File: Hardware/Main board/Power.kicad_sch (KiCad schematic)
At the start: 14 parts, among them U5 AP7361C-33E, U6 AP7361C-33E, U7 AP7361C-33E, U8 AP7361C-33E, U9 TPM8837C

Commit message: Part selection
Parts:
- U5, U6, U7, U8: JLCPCB Part # (none) -> C500795; LCSC Part # (none) -> C500795
- U9: JLCPCB Part # (none) -> C7436831; LCSC Part # (none) -> C7436831
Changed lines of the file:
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@@
+			)
+		)
+		(property "JLCPCB Part #" "C500795"
+			(at 222.25 54.61 0)
+			(effects
+				(font
+					(size 1.27 1.27)
+				)
+				(hide yes)
+			)
+		)
+		(property "LCSC Part #" "C500795"
+			(at 222.25 54.61 0)
+			(effects
+				(font
+					(size 1.27 1.27)
+				)
+				(hide yes)
 			)
 		)
@@
 			)
 		)
+		(property "JLCPCB Part #" "C500795"
+			(at 168.91 64.77 0)
+			(effects
+				(font
+					(size 1.27 1.27)
+				)
+				(hide yes)
+			)
+		)
+		(property "LCSC Part #" "C500795"
+			(at 168.91 64.77 0)
+			(effects
+				(font
+					(size 1.27 1.27)
+				)
+				(hide yes)
+			)
+		)
 		(pin "3"
 		)
@@
 			)
 		)
+		(property "JLCPCB Part #" "C500795"
+			(at 62.23 64.77 0)
+			(effects
+				(font
+					(size 1.27 1.27)
+				)
+				(hide yes)
+			)
+		)
+		(property "LCSC Part #" "C500795"
+			(at 62.23 64.77 0)
+			(effects
+				(font
+					(size 1.27 1.27)
+				)
+				(hide yes)
+			)
+		)
 		(pin "3"
 		)
@@
 			)
 		)
+		(property "JLCPCB Part #" "C7436831"
+			(at 59.69 115.57 0)
+			(effects
+				(font
+					(size 1.27 1.27)
+				)
+				(hide yes)
+			)
+		)
+		(property "LCSC Part #" "C7436831"
+			(at 59.69 115.57 0)
+			(effects
+				(font
+					(size 1.27 1.27)
+				)
+				(hide yes)
+			)
+		)
 		(pin "8"
 		)
@@
 			(at 115.57 64.77 0)
 			(effects
+				(font
+					(size 1.27 1.27)
+				)
+				(hide yes)
+			)
+		)
+		(property "JLCPCB Part #" "C500795"
+			(at 115.57 64.77 0)
+			(effects
+				(font
+					(size 1.27 1.27)
+				)
+				(hide yes)
+			)
+		)
+		(property "LCSC Part #" "C500795"
+			(at 115.57 64.77 0)
+			(effects

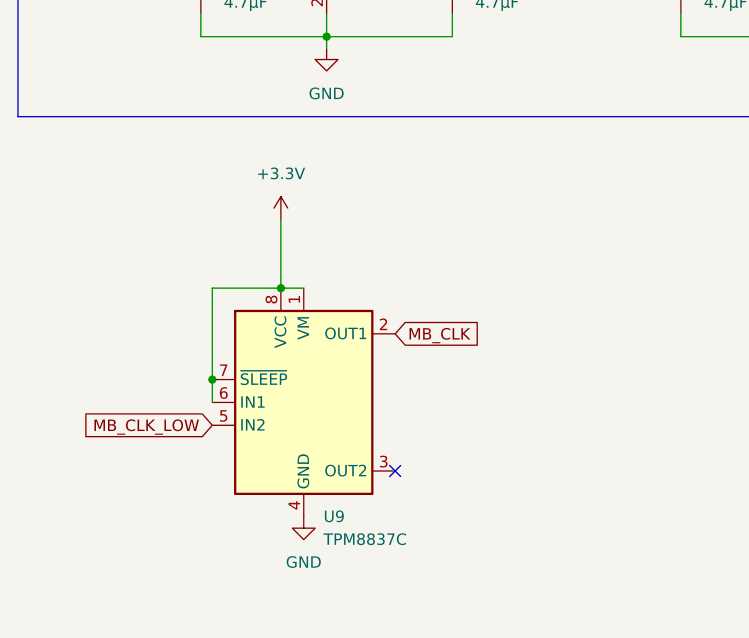
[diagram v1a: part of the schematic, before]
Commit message: Reworking BMS
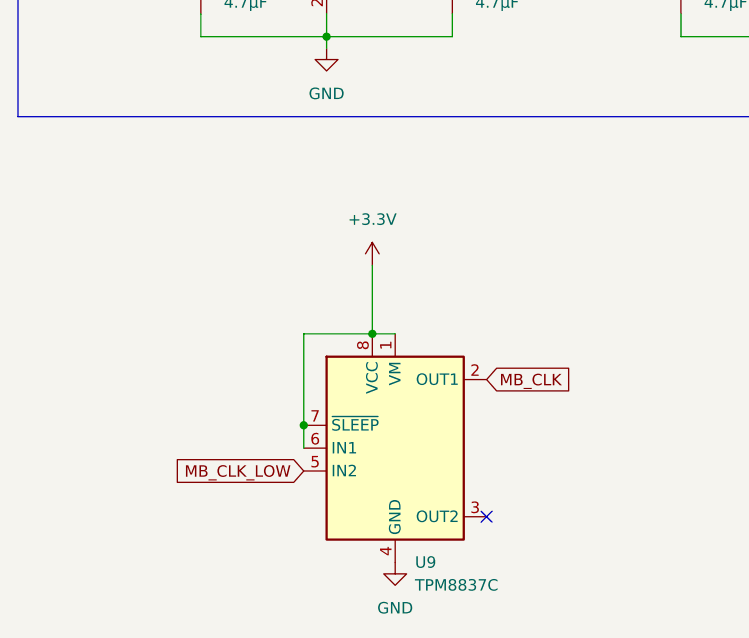
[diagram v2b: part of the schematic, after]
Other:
- moved on the sheet: U9
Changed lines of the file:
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@@
 	(paper "A4")
 	(junction
-		(at 49.53 113.03)
+		(at 59.69 118.11)
 		(diameter 0)
 		(color 0 0 0 0)
@@
 	)
 	(junction
-		(at 57.15 102.87)
+		(at 67.31 107.95)
 		(diameter 0)
 		(color 0 0 0 0)
@@
 	)
 	(no_connect
-		(at 69.85 123.19)
+		(at 80.01 128.27)
 	)
 	(wire
@@
 	(wire
 		(pts
-			(xy 49.53 113.03) (xy 49.53 115.57)
+			(xy 59.69 118.11) (xy 59.69 120.65)
 		)
 		(stroke
@@
 	(wire
 		(pts
-			(xy 57.15 95.25) (xy 57.15 102.87)
+			(xy 67.31 100.33) (xy 67.31 107.95)
 		)
 		(stroke
@@
 	(wire
 		(pts
-			(xy 57.15 102.87) (xy 59.69 102.87)
+			(xy 67.31 107.95) (xy 69.85 107.95)
 		)
 		(stroke
@@
 	(wire
 		(pts
-			(xy 49.53 102.87) (xy 49.53 113.03)
+			(xy 59.69 107.95) (xy 59.69 118.11)
 		)
 		(stroke
@@
 	(wire
 		(pts
-			(xy 57.15 102.87) (xy 49.53 102.87)
+			(xy 67.31 107.95) (xy 59.69 107.95)
 		)
 		(stroke
@@
 	(global_label "MB_CLK_LOW"
 		(shape input)
-		(at 49.53 118.11 180)
+		(at 59.69 123.19 180)
 		(fields_autoplaced yes)
 		(effects
@@
 		)
 		(property "Intersheetrefs" "${INTERSHEET_REFS}"
-			(at 34.5101 118.11 0)
+			(at 44.6701 123.19 0)
 			(effects
 				(font
@@
 	(global_label "MB_CLK"
 		(shape input)
-		(at 69.85 107.95 0)
+		(at 80.01 113.03 0)
 		(fields_autoplaced yes)
 		(effects
@@
 		)
 		(property "Intersheetrefs" "${INTERSHEET_REFS}"
-			(at 80.0923 107.95 0)
+			(at 90.2523 113.03 0)
 			(effects
 				(font
@@
 			)
 		)
+		(property "Design guide" ""
+			(at 101.6 69.85 0)
+			(effects
+				(font
+					(size 1.27 1.27)
+				)
+				(hide yes)
+			)
+		)
 		(pin "1"
 		)
@@
 			)
 		)
+		(property "Design guide" ""
+			(at 236.22 59.69 0)
+			(effects
+				(font
+					(size 1.27 1.27)
+				)
+				(hide yes)
+			)
+		)
 		(pin "1"
 		)
@@
 		)
 		(property "LCSC Part #" "C500795"
+			(at 222.25 54.61 0)
+			(effects
+				(font
+					(size 1.27 1.27)
+				)
+				(hide yes)
+			)
+		)
+		(property "Design guide" ""
 			(at 222.25 54.61 0)
 			(effects
@@
 			)
 		)
+		(property "Design guide" ""
+			(at 76.2 69.85 0)
+			(effects
+				(font
+					(size 1.27 1.27)
+				)
+				(hide yes)
+			)
+		)
 		(pin "1"
 		)
@@
 			)
 		)
+		(property "Design guide" ""
+			(at 48.26 69.85 0)
+			(effects
+				(font
+					(size 1.27 1.27)
+				)
+				(hide yes)
+			)
+		)
 		(pin "1"
 		)
@@
 	(symbol
 		(lib_id "power:+3.3V")
-		(at 57.15 95.25 0)
+		(at 67.31 100.33 0)
 		(unit 1)
 		(exclude_from_sim no)
@@
 		(fields_autoplaced yes)
 		(property "Reference" "#PWR044"
-			(at 57.15 99.06 0)
+			(at 67.31 104.14 0)
 			(effects
 				(font
@@
 		)
 		(property "Value" "+3.3V"
-			(at 57.15 90.17 0)
+			(at 67.31 95.25 0)
 			(effects
 				(font
@@
 		)
 		(property "Footprint" ""
-			(at 57.15 95.25 0)
+			(at 67.31 100.33 0)
 			(effects
 				(font
@@
 		)
 		(property "Datasheet" ""
-			(at 57.15 95.25 0)
+			(at 67.31 100.33 0)
 			(effects
 				(font
@@
 		)
 		(property "Description" "Power symbol creates a global label with name \"+3.3V\""
-			(at 57.15 95.25 0)
+			(at 67.31 100.33 0)
 			(effects
 				(font
@@
 			)
 		)
+		(property "Design guide" ""
+			(at 48.26 49.53 0)
+			(effects
+				(font
+					(size 1.27 1.27)
+				)
+				(hide yes)
+			)
+		)
 		(pin "1"
 		)
@@
 			)
 		)
+		(property "Design guide" ""
+			(at 208.28 59.69 0)
+			(effects
+				(font
+					(size 1.27 1.27)
+				)
+				(hide yes)
+			)
+		)
 		(pin "1"
 		)
@@
 			)
 		)
+		(property "Design guide" ""
+			(at 168.91 64.77 0)
+			(effects
+				(font
+					(size 1.27 1.27)
+				)
+				(hide yes)
+			)
+		)
 		(pin "3"
 		)
@@
 			)
 		)
+		(property "Design guide" ""
+			(at 182.88 69.85 0)
+			(effects
+				(font
+					(size 1.27 1.27)
+				)
+				(hide yes)
+			)
+		)
 		(pin "1"
 		)
@@
 			)
 		)
+		(property "Design guide" ""
+			(at 62.23 64.77 0)
+			(effects
+				(font
+					(size 1.27 1.27)
+				)
+				(hide yes)
+			)
+		)
 		(pin "3"
 		)
@@
 	(symbol
 		(lib_id "power:GND")
-		(at 59.69 128.27 0)
+		(at 69.85 133.35 0)
 		(unit 1)
 		(exclude_from_sim no)
@@
 		(fields_autoplaced yes)
 		(property "Reference" "#PWR045"
-			(at 59.69 134.62 0)
+			(at 69.85 139.7 0)
 			(effects
 				(font
@@
 		)
 		(property "Value" "GND"
-			(at 59.69 133.35 0)
+			(at 69.85 138.43 0)
 			(effects
 				(font
@@
 		)
 		(property "Footprint" ""
-			(at 59.69 128.27 0)
+			(at 69.85 133.35 0)
 			(effects
 				(font
@@
 		)
 		(property "Datasheet" ""
-			(at 59.69 128.27 0)
+			(at 69.85 133.35 0)
 			(effects
 				(font
@@
 		)
 		(property "Description" "Power symbol creates a global label with name \"GND\" , ground"
-			(at 59.69 128.27 0)
+			(at 69.85 133.35 0)
 			(effects
 				(font
@@
 			)
 		)
+		(property "Design guide" ""
+			(at 129.54 69.85 0)
+			(effects
+				(font
+					(size 1.27 1.27)
+				)
+				(hide yes)
+			)
+		)
 		(pin "1"
 		)
@@
 	(symbol
 		(lib_id "Driver_Motor:DRV8837C")
-		(at 59.69 115.57 0)
+		(at 69.85 120.65 0)
 		(unit 1)
 		(exclude_from_sim no)
@@
 		(dnp no)
 		(property "Reference" "U9"
-			(at 61.8841 128.27 0)
+			(at 72.0441 133.35 0)
 			(effects
 				(font
@@
 		)
 		(property "Value" "TPM8837C"
-			(at 61.8841 130.81 0)
+			(at 72.0441 135.89 0)
 			(effects
 				(font
@@
 		)
 		(property "Footprint" "Package_SO:SOIC-8_3.9x4.9mm_P1.27mm"
-			(at 59.69 137.16 0)
+			(at 69.85 142.24 0)
 			(effects
 				(font
@@
 		)
 		(property "Datasheet" "http://www.ti.com/lit/ds/symlink/drv8837c.pdf"
-			(at 59.69 115.57 0)
+			(at 69.85 120.65 0)
 			(effects
 				(font
@@
 		)
 		(property "Description" "H-Bridge driver, 1A, Low Voltage, PWM input, WSON-8"
-			(at 59.69 115.57 0)
+			(at 69.85 120.65 0)
 			(effects
 				(font
@@
 		)
 		(property "JLCPCB Part #" "C7436831"
-			(at 59.69 115.57 0)
+			(at 69.85 120.65 0)
 			(effects
 				(font
@@
 		)
 		(property "LCSC Part #" "C7436831"
-			(at 59.69 115.57 0)
+			(at 69.85 120.65 0)
+			(effects
+				(font
+					(size 1.27 1.27)
+				)
+				(hide yes)
+			)
+		)
+		(property "Design guide" ""
+			(at 69.85 120.65 0)
 			(effects
 				(font
@@
 			)
 		)
+		(property "Design guide" ""
+			(at 154.94 69.85 0)
+			(effects
+				(font
+					(size 1.27 1.27)
+				)
+				(hide yes)
+			)
+		)
 		(pin "1"
 		)
@@
 			(at 115.57 64.77 0)
 			(effects
+				(font
+					(size 1.27 1.27)
+				)
+				(hide yes)
+			)
+		)
+		(property "Design guide" ""
+			(at 115.57 64.77 0)
+			(effects
